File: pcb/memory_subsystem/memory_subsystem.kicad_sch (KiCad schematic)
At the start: 15 parts, among them J1 CLK, J2 Addr In, J3 Data In, J4 Word In, J5 Power, SW1 RUN, SW2 HLT, SW3 HLT Word, SW4 SW_DIP_x01

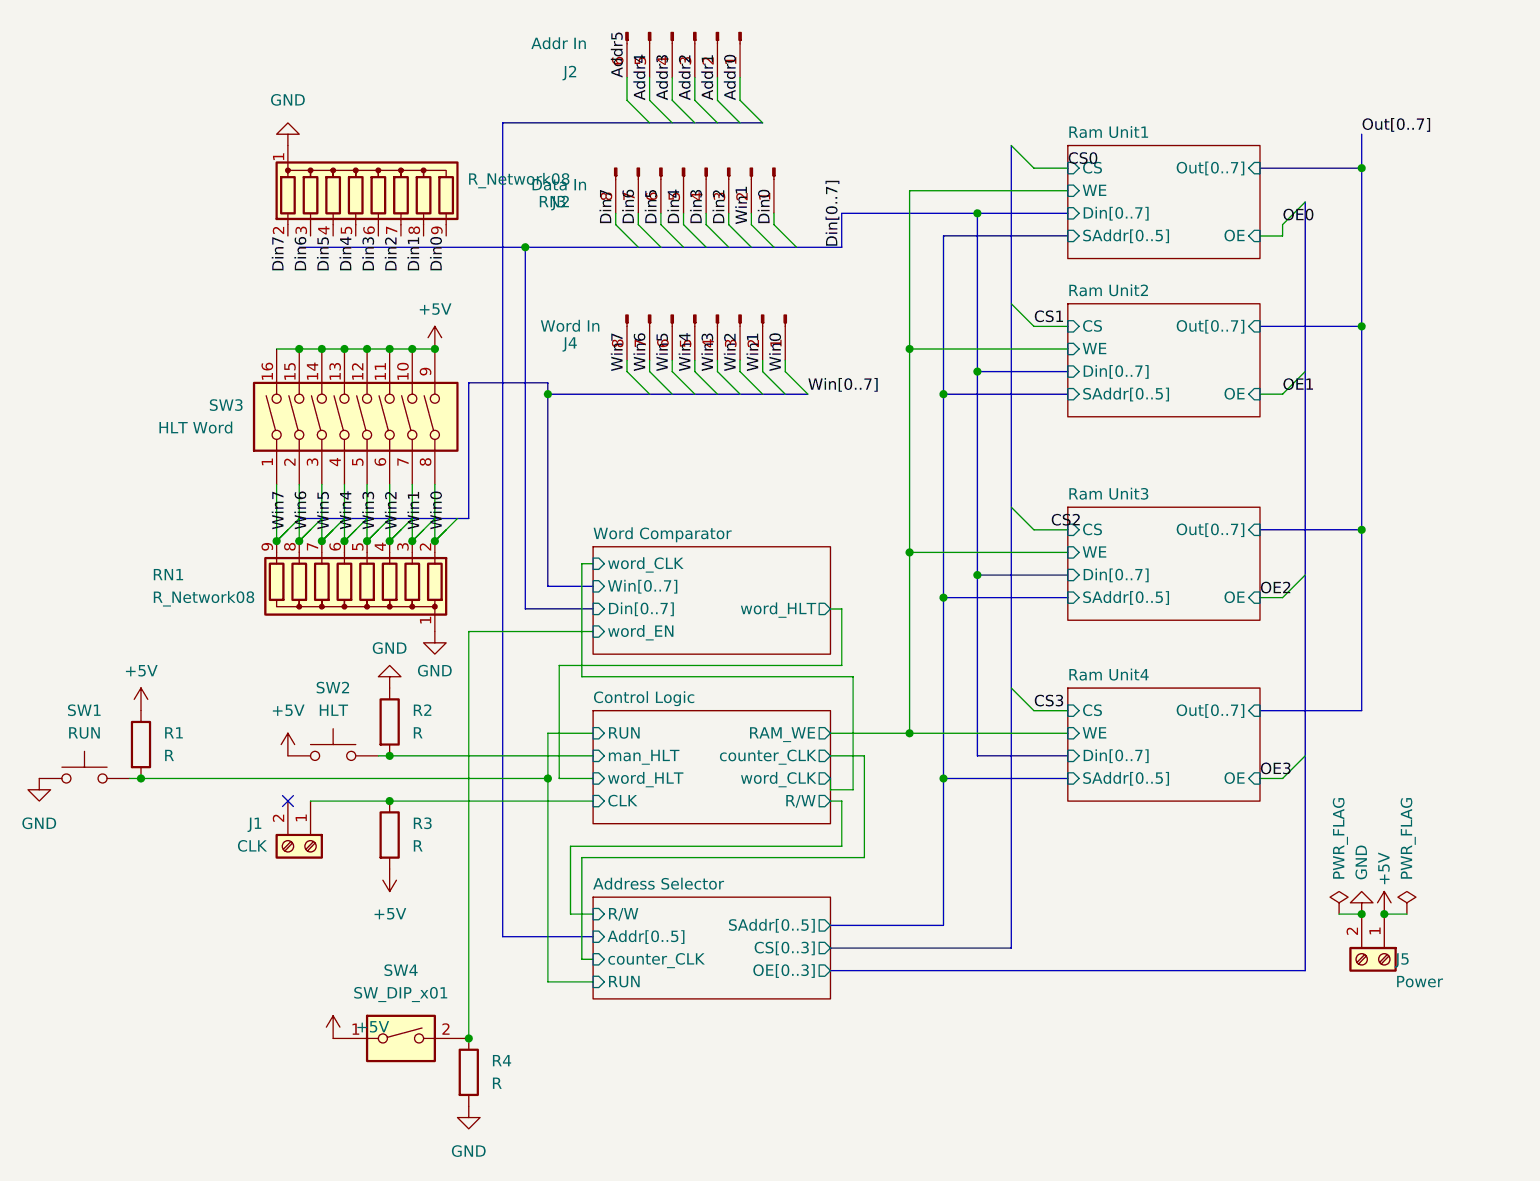
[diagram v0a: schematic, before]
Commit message: Tracks finished
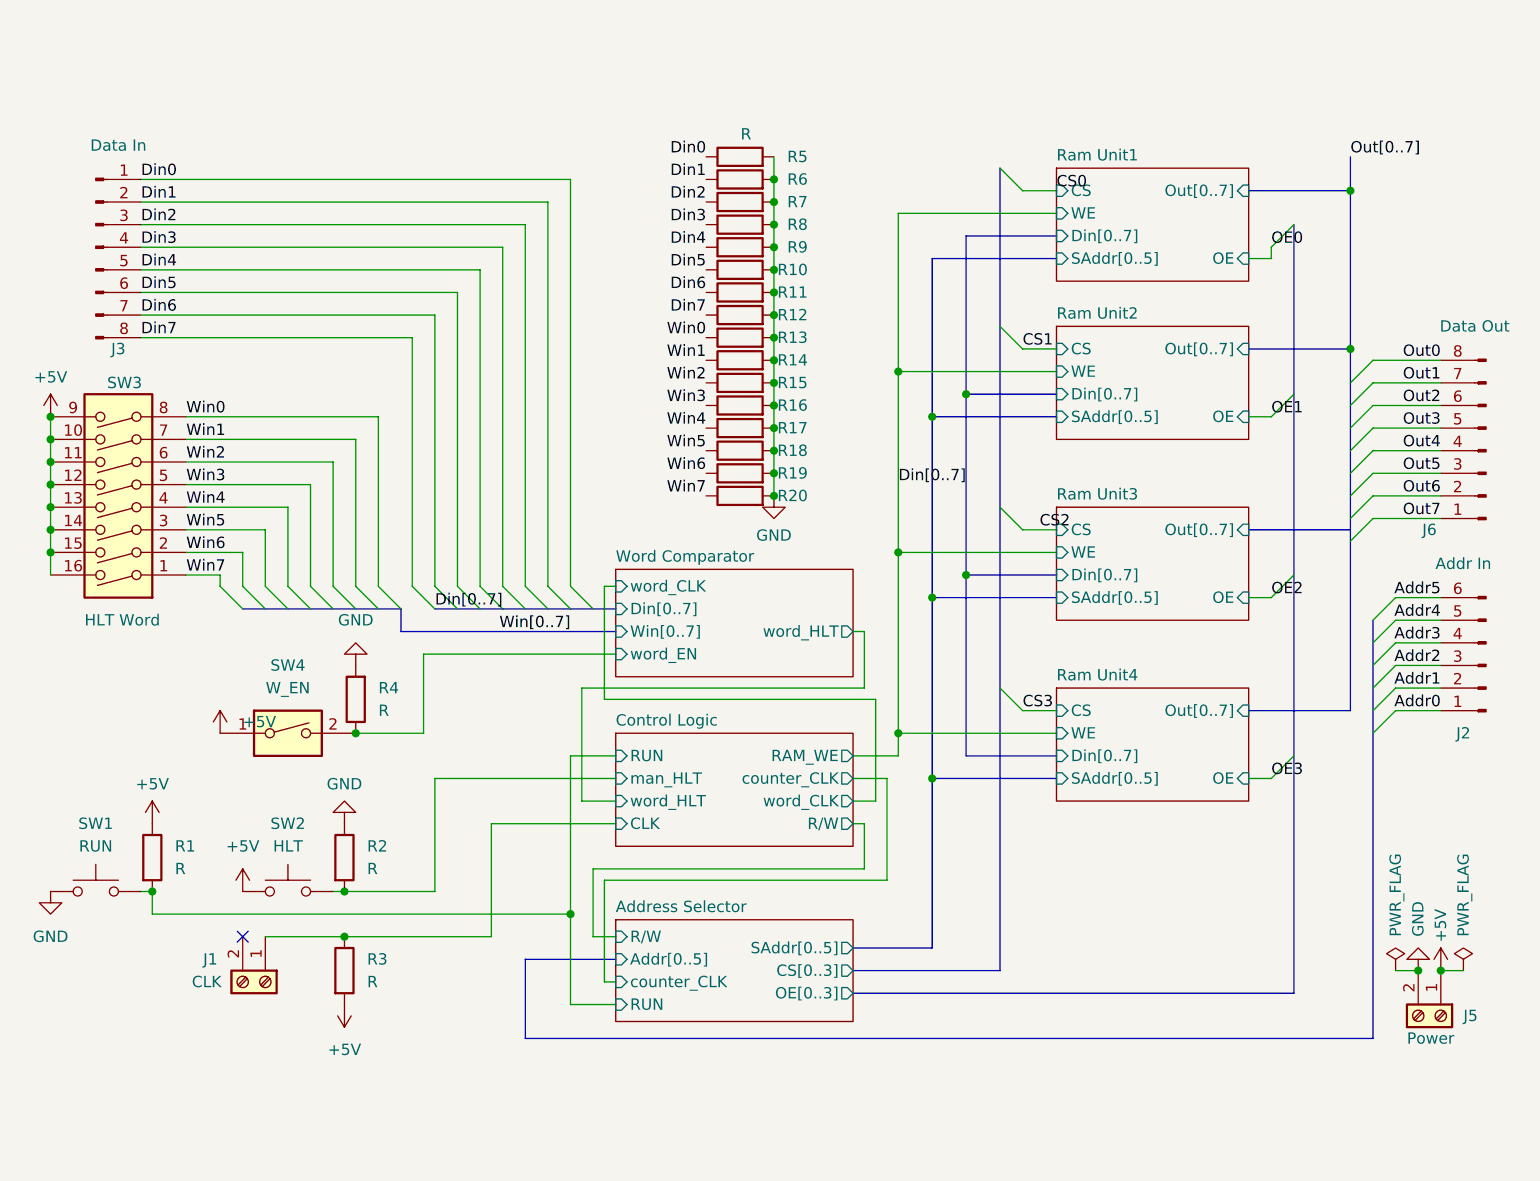
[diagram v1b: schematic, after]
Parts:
- removed J4: Word In, symbol Connector:Conn_01x08_Pin
- removed RN1, RN2: R_Network08, Resistor_THT:R_Array_SIP9, symbol Device:R_Network08
- added J6: Data Out, Connector_PinHeader_2.54mm:PinHeader_1x08_P2.54mm_Vertical, symbol Connector:Conn_01x08_Pin
- added R10, R11, R12, R13, R14, R15, R16, R17, R18, R19, R20, R5, R6, R7, R8, R9: R, Resistor_SMD:R_0805_2012Metric_Pad1.20x1.40mm_HandSolder, symbol Device:R
- J1, J5: footprint (none) -> TerminalBlock_Phoenix:TerminalBlock_Phoenix_MKDS-1,5-2_1x02_P5.00mm_Horizontal
- J2: footprint (none) -> Connector_PinHeader_2.54mm:PinHeader_1x06_P2.54mm_Vertical
- J3: footprint (none) -> Connector_PinHeader_2.54mm:PinHeader_1x08_P2.54mm_Vertical
- R1, R2, R3, R4: footprint (none) -> Resistor_SMD:R_0805_2012Metric_Pad1.20x1.40mm_HandSolder
- SW1, SW2: footprint (none) -> Button_Switch_THT:SW_TH_Tactile_Omron_B3F-100x
- SW3: footprint (none) -> Button_Switch_THT:SW_DIP_SPSTx08_Slide_9.78x22.5mm_W7.62mm_P2.54mm
- SW4: value SW_DIP_x01 -> W_EN; footprint (none) -> Button_Switch_THT:SW_DIP_SPSTx01_Slide_9.78x4.72mm_W7.62mm_P2.54mm
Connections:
- net Din0: now also R5.1
- net Din1: now also J3.2 (Pin_2), R6.1
- net Din2: now also R7.1
- net Din3: now also R8.1
- net Din4: now also R9.1
- net Din5: now also R10.1
- net Din6: now also R11.1
- net Din7: now also R12.1
- net GND: now also R10.2, R11.2, R12.2, R13.2, R14.2, R15.2, R16.2, R17.2, R18.2, R19.2, R20.2, R5.2, R6.2, R7.2, R8.2, R9.2
- net Win0: now also R13.1
- net Win1: now also R14.1; no longer J3.2 (Pin_2)
- net Win2: now also R15.1
- net Win3: now also R16.1
- net Win4: now also R17.1
- net Win5: now also R18.1
- net Win6: now also R19.1
- net Win7: now also R20.1
- new net Out0: J6.8 (Pin_8)
- new net Out1: J6.7 (Pin_7)
- new net Out2: J6.6 (Pin_6)
- new net Out3: J6.5 (Pin_5)
- new net Out4: J6.4 (Pin_4)
- new net Out5: J6.3 (Pin_3)
- new net Out6: J6.2 (Pin_2)
- new net Out7: J6.1 (Pin_1)
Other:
- moved on the sheet: J1, J2, J3, J5, R1, R2, R3, R4, SW1, SW2, SW3, SW4
